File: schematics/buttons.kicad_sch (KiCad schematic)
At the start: 25 parts, among them SW2 SW_SPST, SW3 SW_SPST, SW4 SW_SPST, SW5 SW_SPST, SW6 SW_SPST, SW7 SW_SPST, SW8 SW_SPST, SW9 SW_SPST, U2 ADS1115IDGS

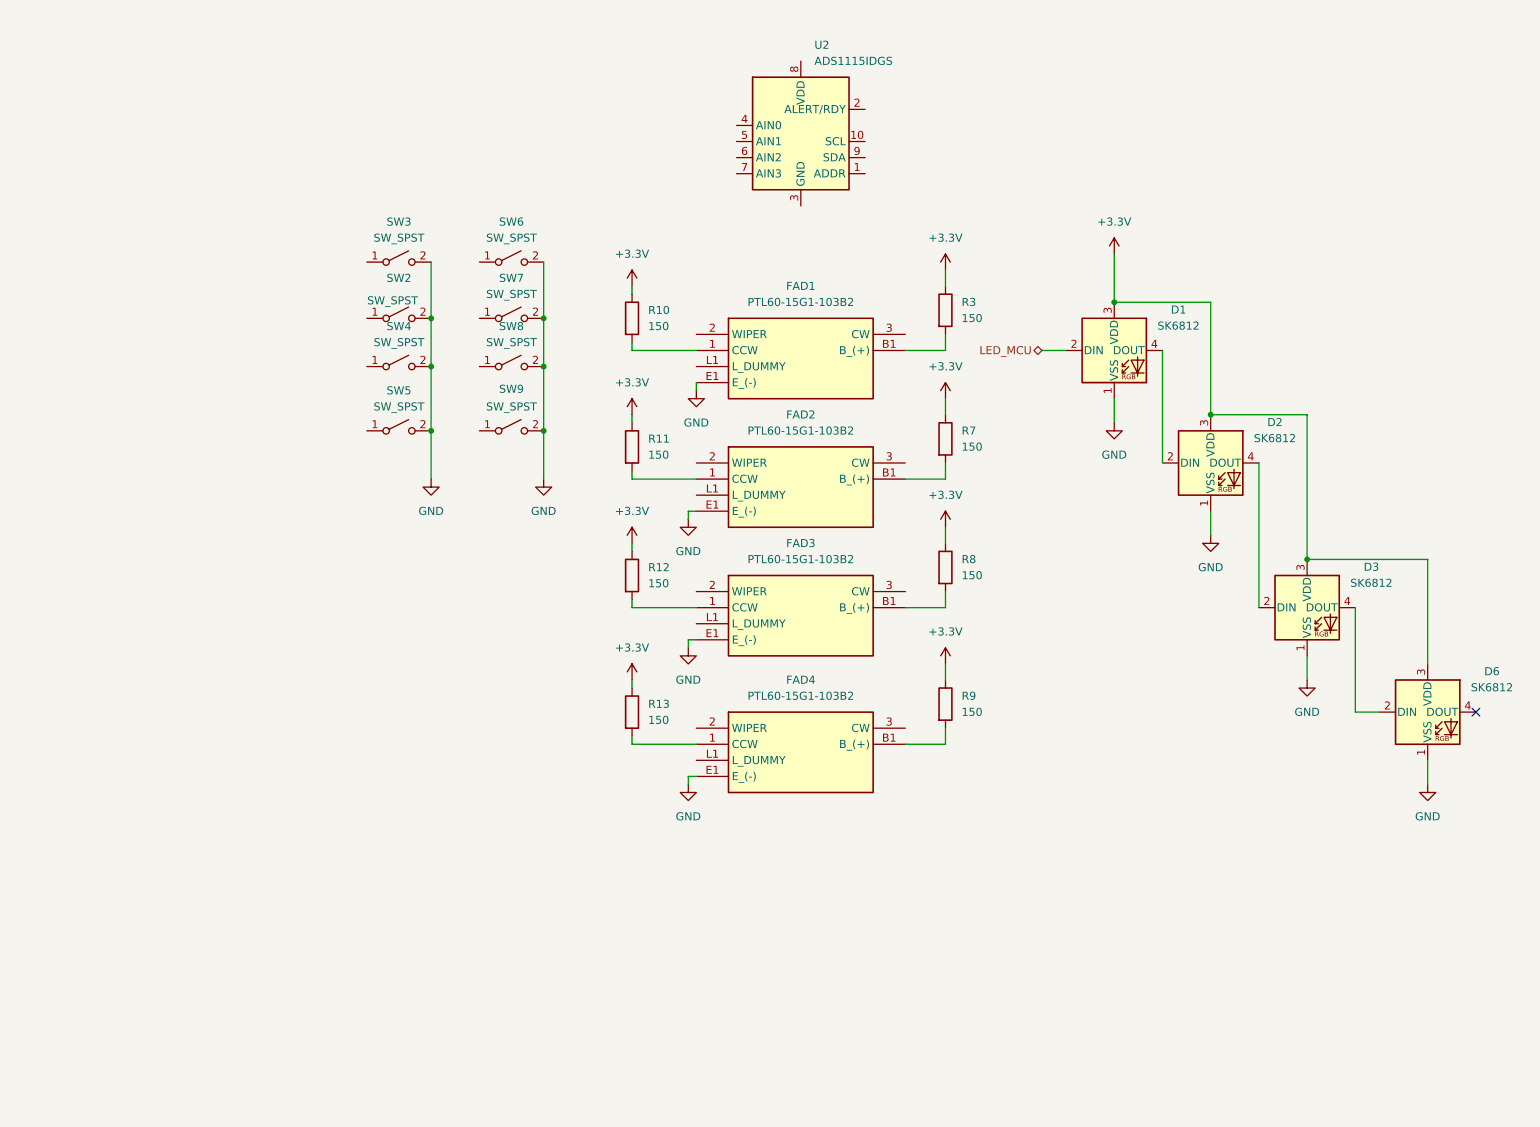
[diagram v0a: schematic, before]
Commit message: Update README
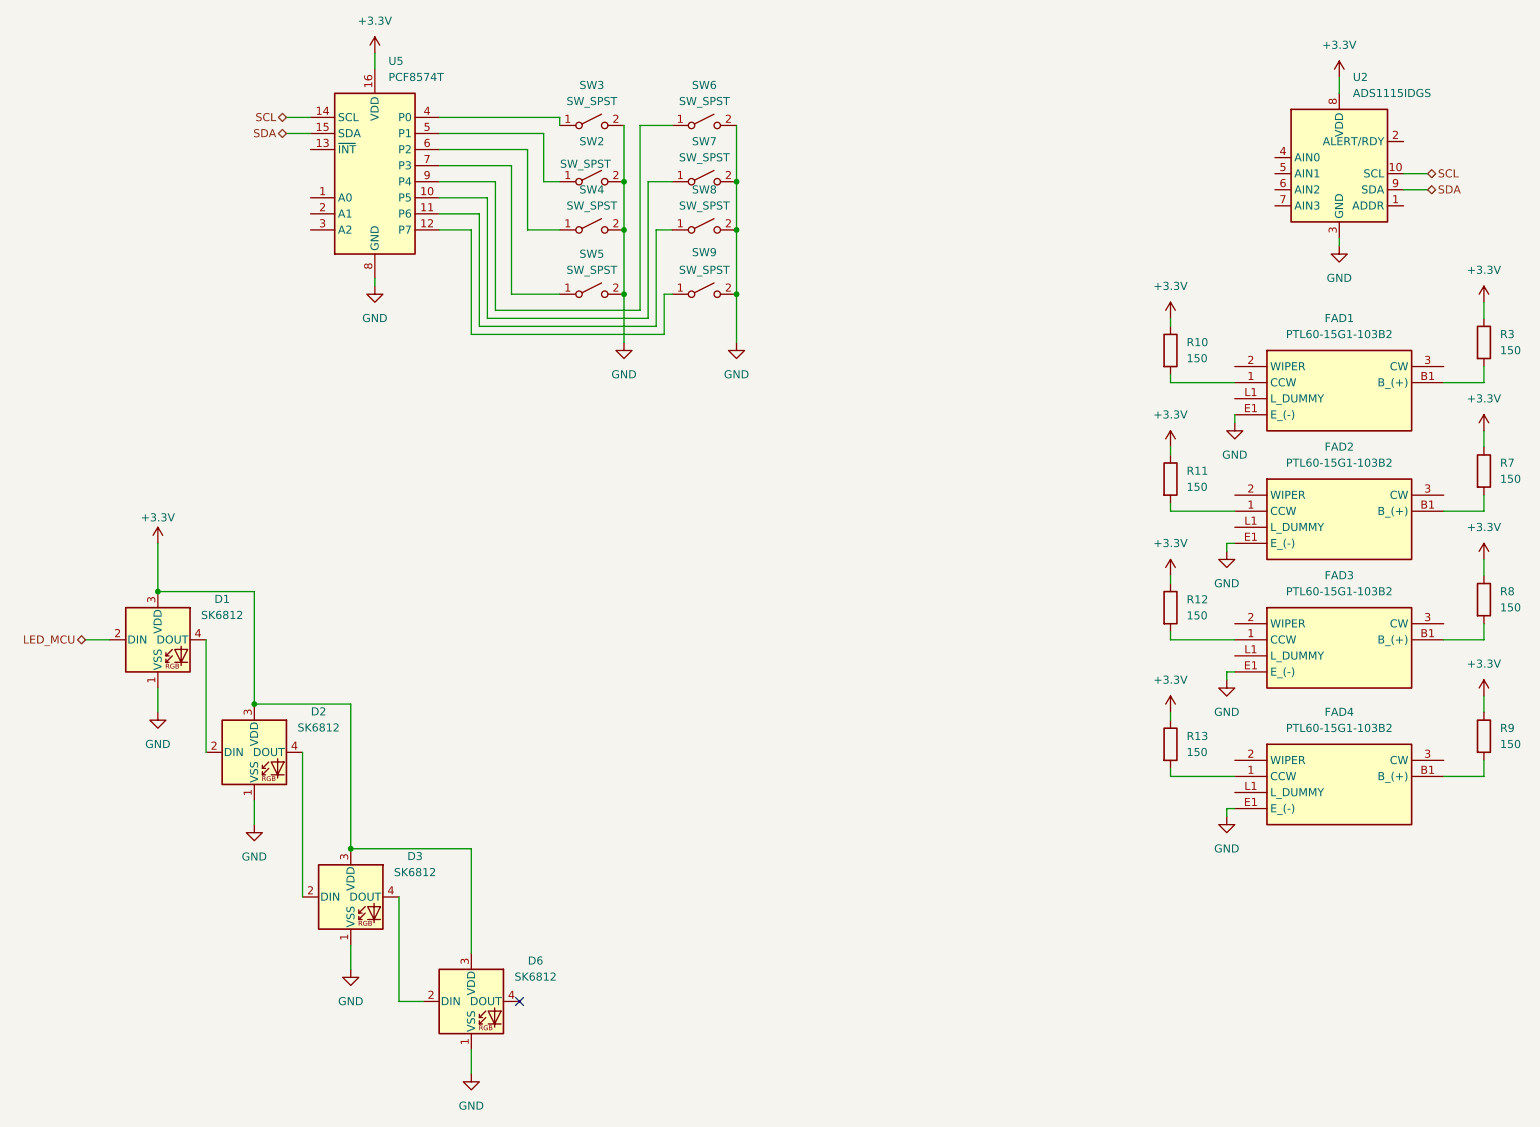
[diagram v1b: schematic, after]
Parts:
- added U5: PCF8574T, Package_SO:SOIC-16W_7.5x10.3mm_P1.27mm, symbol Interface_Expansion:PCF8574T
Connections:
- net +3.3V: now also U2.8 (VDD), U5.16 (VDD)
- net GND: now also U2.3 (GND), U5.8 (GND)
- net at SW5.1 (A): now also U5.7 (P3)
- net SCL: now reaches U2.10 (SCL)
- net SCL: now also U5.14 (SCL)
- net SDA: now reaches U2.9 (SDA)
- net SDA: now also U5.15 (SDA)
- net at SW9.1 (A): now also U5.12 (P7)
- net at SW3.1 (A): now also U5.4 (P0)
- net at SW4.1 (A): now also U5.6 (P2)
- net at SW6.1 (A): now also U5.9 (P4)
- net at SW2.1 (A): now also U5.5 (P1)
- net at SW7.1 (A): now also U5.10 (P5)
- net at SW8.1 (A): now also U5.11 (P6)
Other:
- moved on the sheet: D1, D2, D3, D6, FAD1, FAD2, FAD3, FAD4, R10, R11, R12, R13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
